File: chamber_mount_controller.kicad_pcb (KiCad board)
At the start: 2 copper layers, 10 parts, among them J1 Conn_01x04, J2 Conn_01x04, J3 Conn_01x02

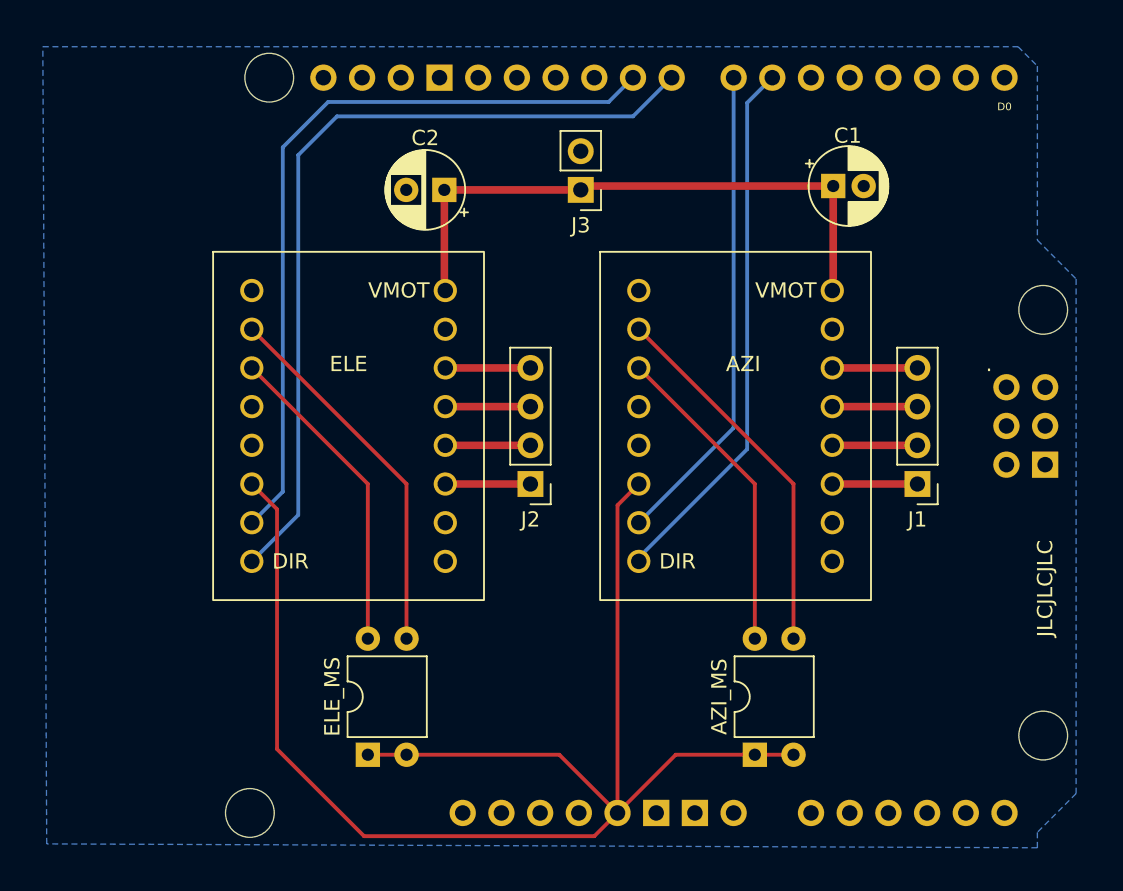
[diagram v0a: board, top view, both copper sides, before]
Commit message: updated files
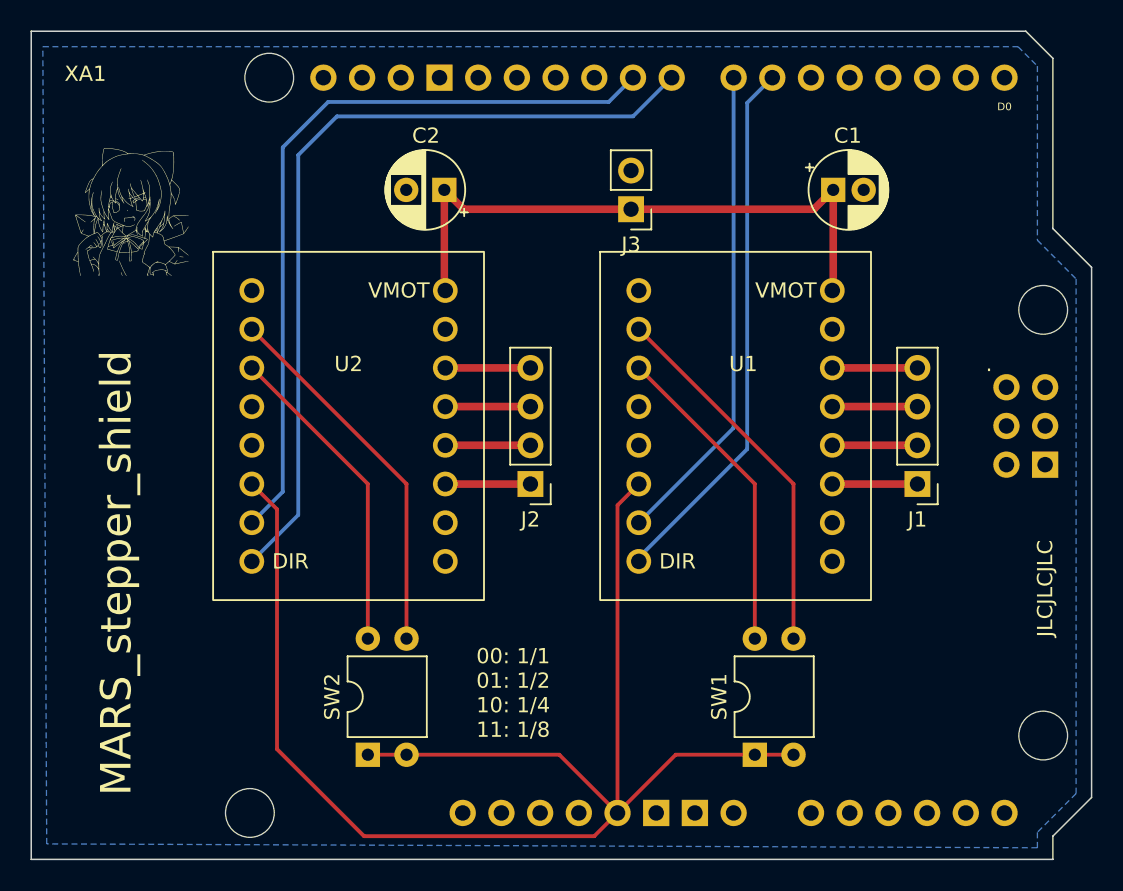
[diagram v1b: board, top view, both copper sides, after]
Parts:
- added G***: LOGO, Library:cirno_logo, F.Cu at (91.2, 54.4)
- moved J3 3.54 mm to (125.2, 54.4)
- moved C1 0.25 mm to (138.5, 53.1)
- renumbered AZI_MS to SW1, ELE_MS to SW2, AZI to U1, ELE to U2
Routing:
- net VCC: track 39.1 -> 40.1 mm
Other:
- board outline added: 69.6 x 54.4 mm
- board text added: "00: 1/1 01: 1/2 10: 1/4 11: 1/8"
- board text added: "MARS_stepper_shield"
